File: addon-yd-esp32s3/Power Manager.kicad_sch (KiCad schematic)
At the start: 33 parts, among them Q1 Q_NMOS_DGS, Q2 Q_NMOS_DGS, Q3 DMP2160U-7, U1 DW01A, U3 TP4056, U4 TLV62565DBVR, U5 SDB628

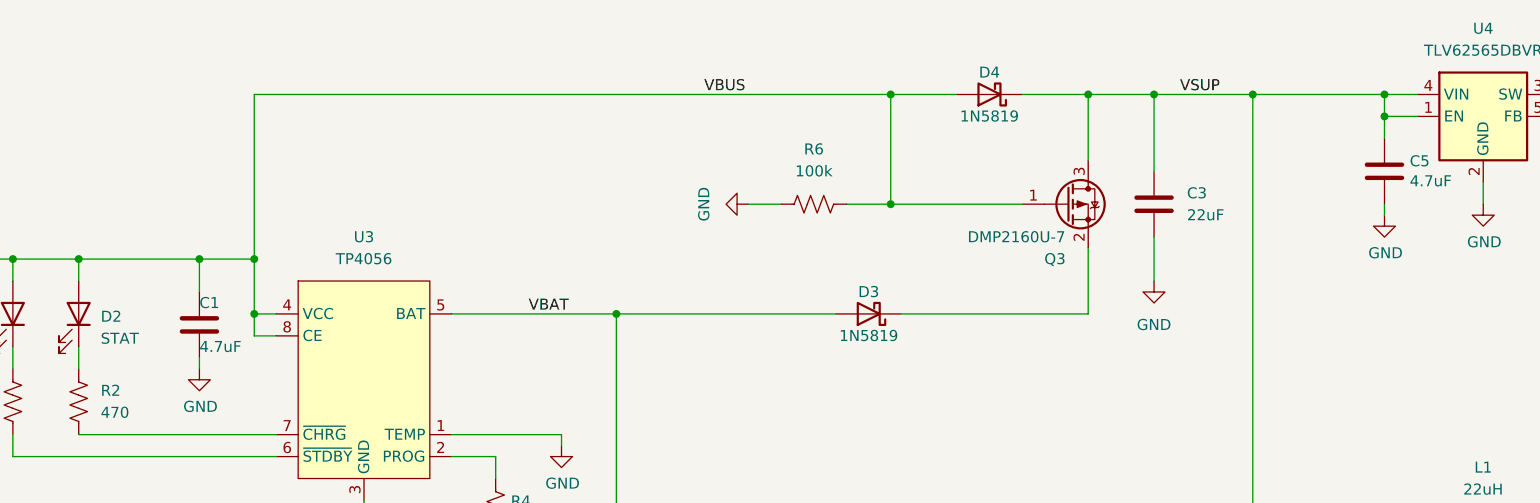
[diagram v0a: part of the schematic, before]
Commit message: completando el diseño
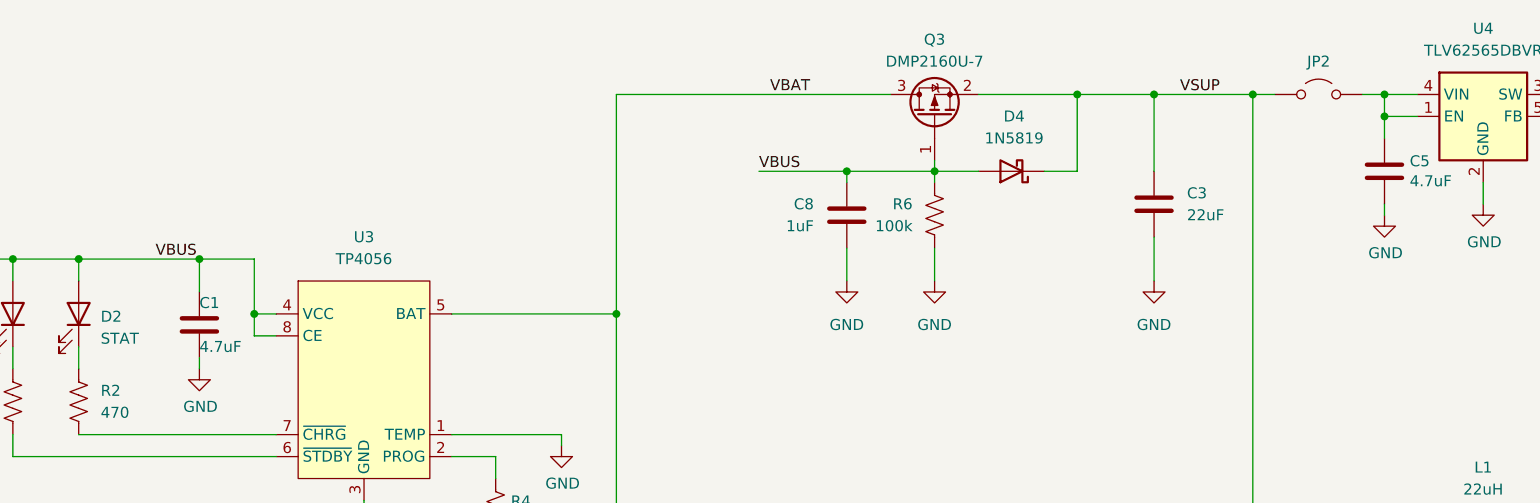
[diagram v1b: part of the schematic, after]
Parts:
- removed D3: 1N5819, Diode_SMD:D_SOD-123, symbol Diode:B120-E3
- added C8: 1uF, Capacitor_SMD:C_0603_1608Metric, symbol Device:C
- added JP2: Jumper_2_Open, Jumper:SolderJumper-2_P1.3mm_Open_TrianglePad1.0x1.5mm, symbol Jumper:Jumper_2_Open
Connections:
- net GND: now also C8.2
- net VBAT: now also Q3.3 (D)
- net VBUS: now also C8.1
- net VSUP: now also Q3.2 (S), JP2.1 (A); no longer C5.1, Q3.3 (D), U4.1 (EN), U4.4 (VIN)
- new net: C5.1, JP2.2 (B), U4.1 (EN), U4.4 (VIN)
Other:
- moved on the sheet: D4, Q3, R6
